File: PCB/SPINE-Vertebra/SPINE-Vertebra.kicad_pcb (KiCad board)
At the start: 2 copper layers, 49 x 49 mm, 75 parts, among them J2 Conn_01x06, J4 Conn_01x06, Q1 NTMFS5C628NLT1G, Q2 NTMFS5C628NLT1G, Q3 NTMFS5C628NLT1G, Q4 NTMFS5C628NLT1G, Q7 VISHAY SI2309CDS-T1-GE3, Q8 Q_NMOS_GSD, U1 ACS724xLCTR-50AB, U2 LM74800QDRRRQ1, U3 SP3485EN, U4 MIC5219-3.3YM5, U5 STM32G030F6Px

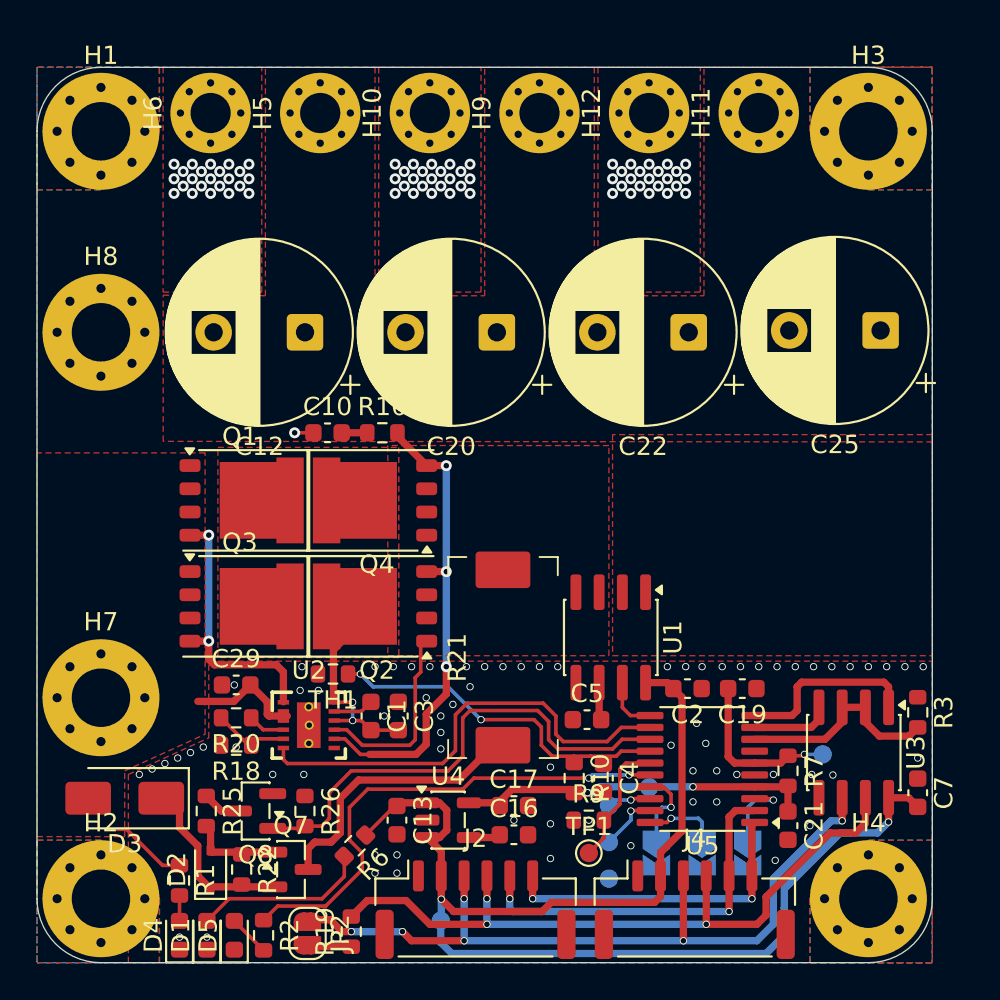
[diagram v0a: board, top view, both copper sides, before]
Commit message: Finish Vertebra
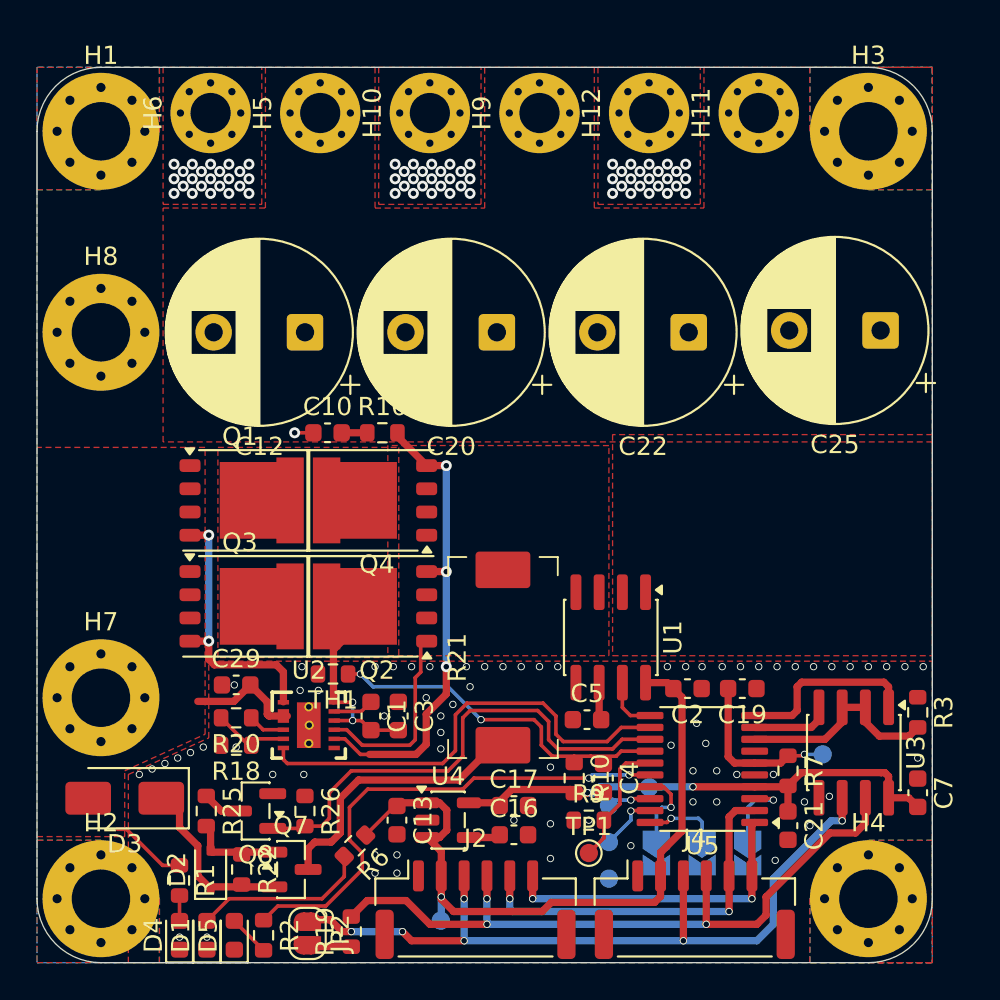
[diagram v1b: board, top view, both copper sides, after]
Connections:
- C7 pad 2: +5V -> +3.3V
- U3 pad 8: +5V -> +3.3V
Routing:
- net +5V: track 72.7 -> 39.3 mm, vias 2 -> 1
- net +3.3V: track 19.6 -> 28.5 mm
